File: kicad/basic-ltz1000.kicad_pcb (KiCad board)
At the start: 2 copper layers, 49.5 x 49.5 mm, 35 parts, among them P1 CONN_1X1, P2 CONN_1X1, P3 CONN_1X1, P4 CONN_1X1, P5 CONN_1X1, Q1 2N3904, U1 LTZ1000A, U2 LT1013

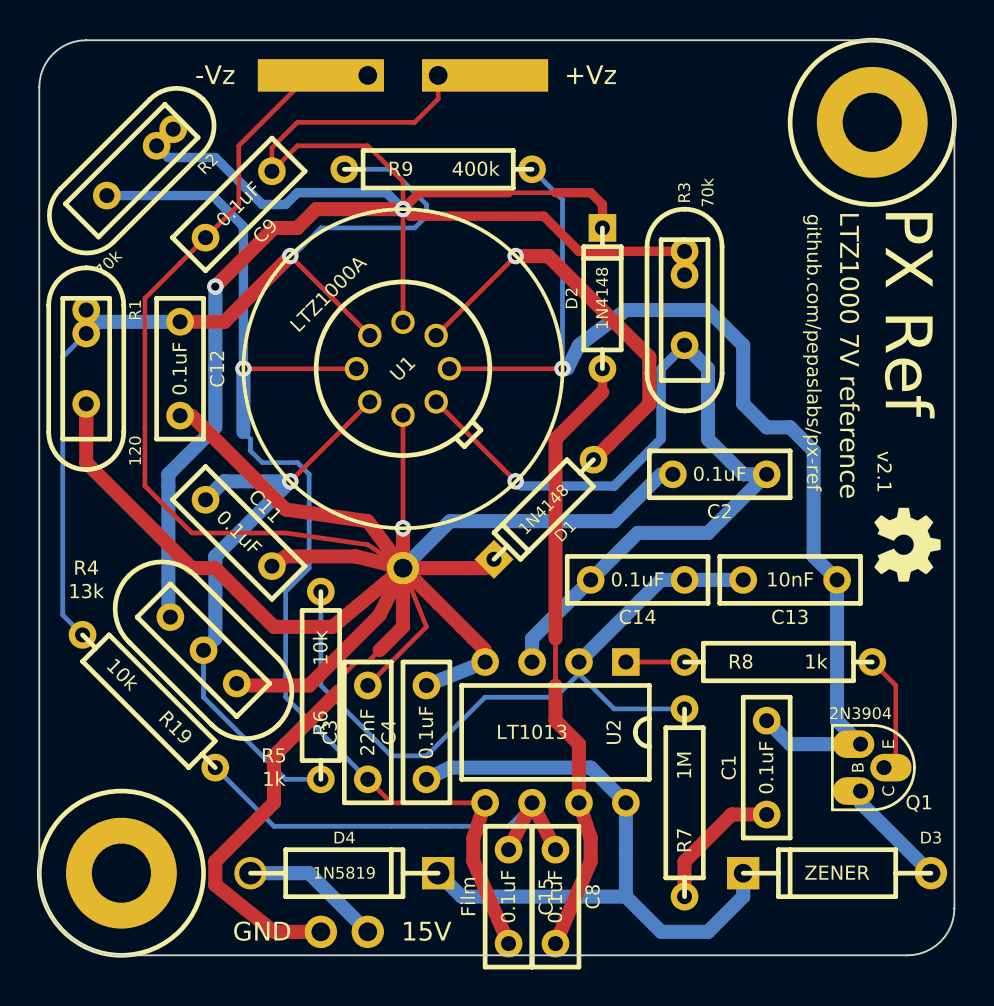
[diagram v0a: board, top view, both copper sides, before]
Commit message: WIP
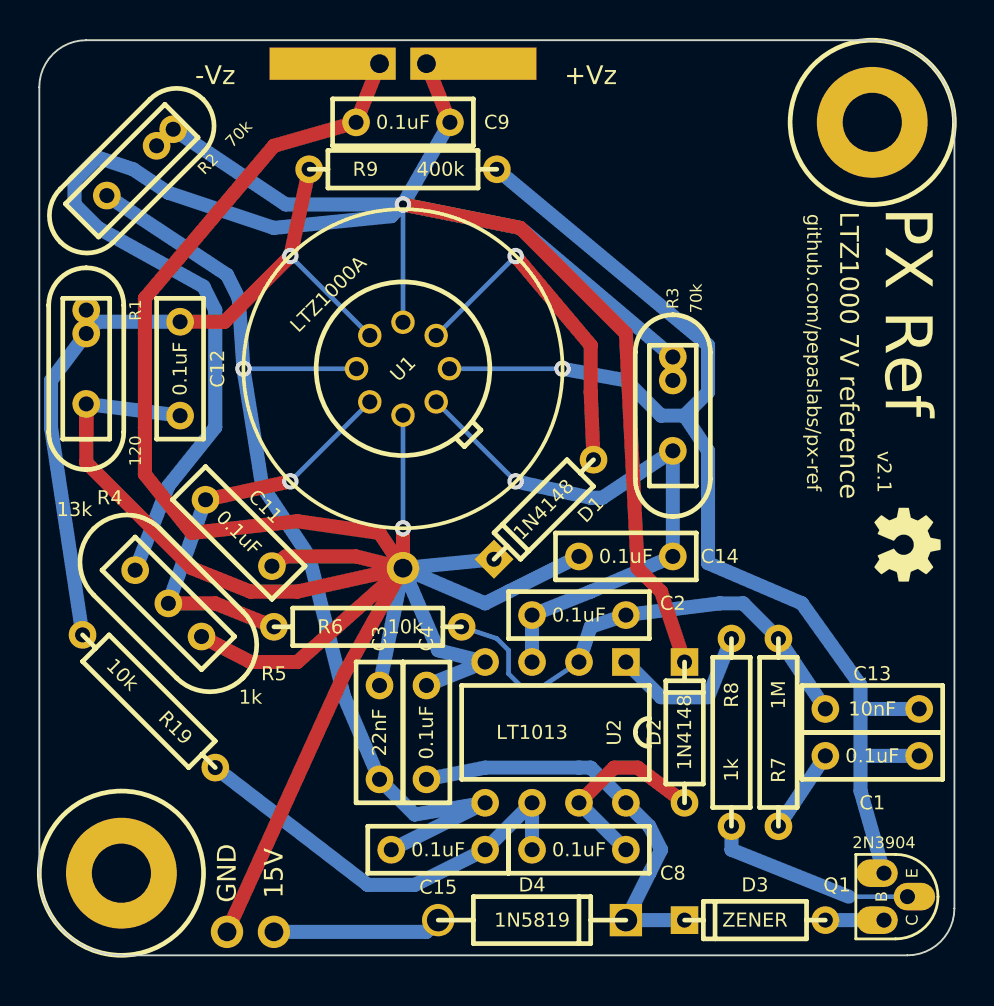
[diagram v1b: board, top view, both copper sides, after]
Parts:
- D3: footprint DIODE_1A_069A_PL -> DIODE_SS_059A_PL
- moved D2 23.9 mm to (233.0, 102.2)
- moved D4 10.5 mm to (224.8, 112.4)
- moved C9 9.94 mm to (217.8, 69.2), turned to 180 degrees
- moved R6 8.64 mm to (210.8, 96.5), turned to 0 degrees
- moved C13 8.28 mm to (243.2, 101.0)
- moved Q1 7.10 mm to (243.8, 109.9)
- moved C2 6.75 mm to (229.9, 92.7)
- moved R7 6.35 mm to (238.1, 107.3)
- moved C1 5.75 mm to (243.2, 103.5), turned to 0 degrees
- moved R3 5.75 mm to (232.4, 83.2)
- moved D3 5.12 mm to (236.9, 112.4)
- moved P1 5.08 mm to (210.8, 113.0)
- moved P4 5.08 mm to (208.3, 113.0)
- moved C15 4.58 mm to (219.7, 108.6), turned to 180 degrees
- moved C14 3.70 mm to (227.3, 95.9)
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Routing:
- net Vz- Sense: track 187.3 -> 162.0 mm
- net 15V: track 47.0 -> 22.3 mm
- net N-0000014: track 33.2 -> 10.7 mm
- net Vz+ Sense: track 106.3 -> 127.2 mm, vias 2 -> 1
- net N-000004: track 47.9 -> 32.3 mm
- net N-0000013: track 41.0 -> 26.3 mm
- net N-0000010: track 32.9 -> 22.7 mm
- net N-0000015: track 51.5 -> 42.1 mm
- net N-000005: track 64.3 -> 55.3 mm
- net H+: track 60.2 -> 69.1 mm
- net N-0000012: track 3.17 -> 8.65 mm
- net N-0000011: track 6.50 -> 11.3 mm
- net N-000009: track 22.4 -> 18.6 mm
- net N-000007: track 6.02 -> 3.18 mm
- net N-0000016: track 7.40 -> 4.58 mm
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
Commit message: v2.1 gerbers
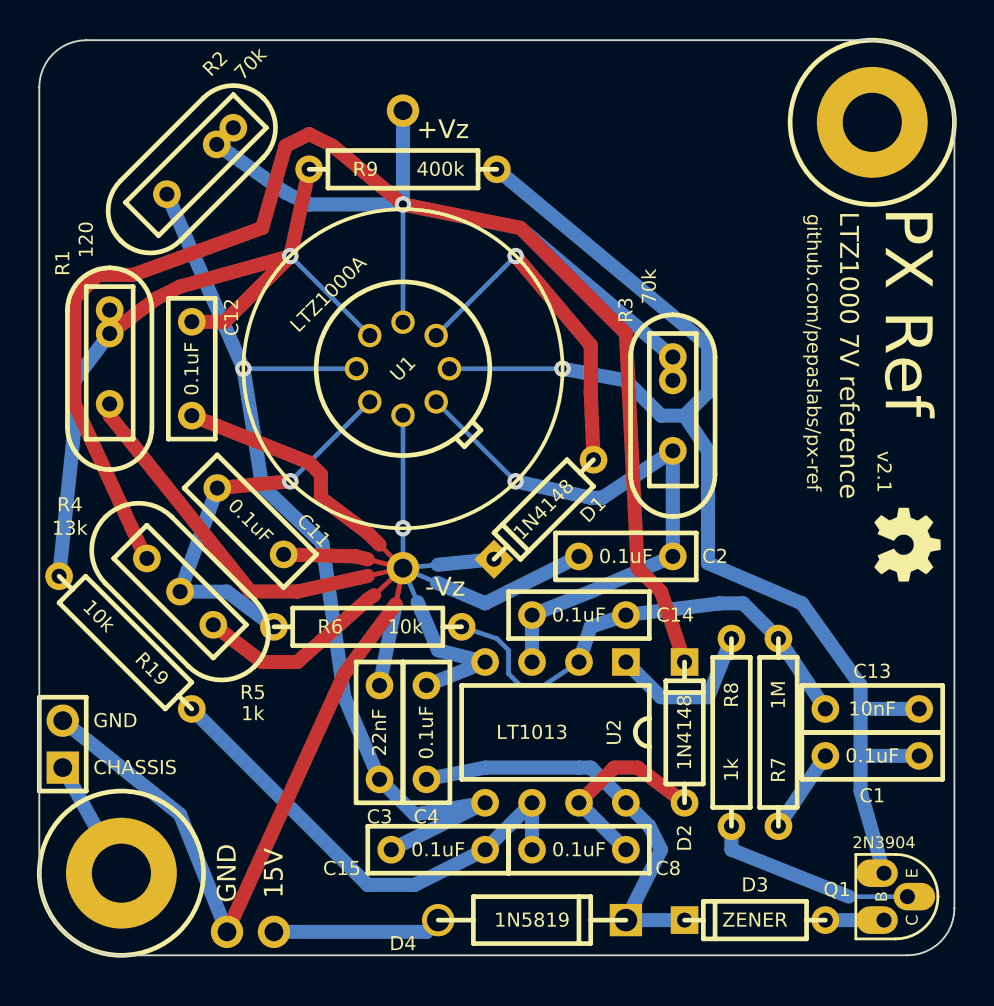
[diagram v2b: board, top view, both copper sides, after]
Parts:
- removed C9: 0.1uF, BOXCAP_01_03_02_059A
- removed the H*** at (202.6, 109.9)
- removed P3: CONN_1X1, 1pin_040_069_strip_2_PL
- added H1: HOLE, hole_M3, F.Cu at (202.6, 109.9)
- added P6: CONN_2X1, SIL-2, F.Cu at (199.4, 104.1)
- P2: footprint 1pin_040_069_strip_2_PL -> 1pin_040_069
- R1, R2, R3: footprint R_BOX_PL -> R_BOX_HERMETIC_PL
- moved R19 3.42 mm to (206.4, 101.0)
- moved P2 2.84 mm to (217.8, 68.6), turned to 0 degrees
- moved R1 2.29 mm to (201.9, 82.5)
- moved R2 2.29 mm to (206.4, 71.8)
- moved R3 1.91 mm to (232.4, 85.1)
- moved R45 0.90 mm to (205.7, 94.6)
- moved C11 0.90 mm to (209.6, 90.8)
- moved C12 0.63 mm to (206.4, 82.5)
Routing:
- net Vz- Sense: track 162.0 -> 137.2 mm
- net Vz+ Sense: track 127.2 -> 113.9 mm
- net CHASSIS: track 0.00 -> 6.54 mm
- net N-000008: track 23.3 -> 26.4 mm
- net N-000007: track 55.3 -> 52.9 mm
- net N-0000016: track 42.1 -> 43.7 mm
- net N-0000011: track 22.7 -> 21.7 mm
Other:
- board text added: "CHASSIS"
